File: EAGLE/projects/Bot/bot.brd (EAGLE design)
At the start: 124.3 x 90 mm, 17 parts, among them IC1 7805T, U3 ARDUINO_SHIELDLABEL

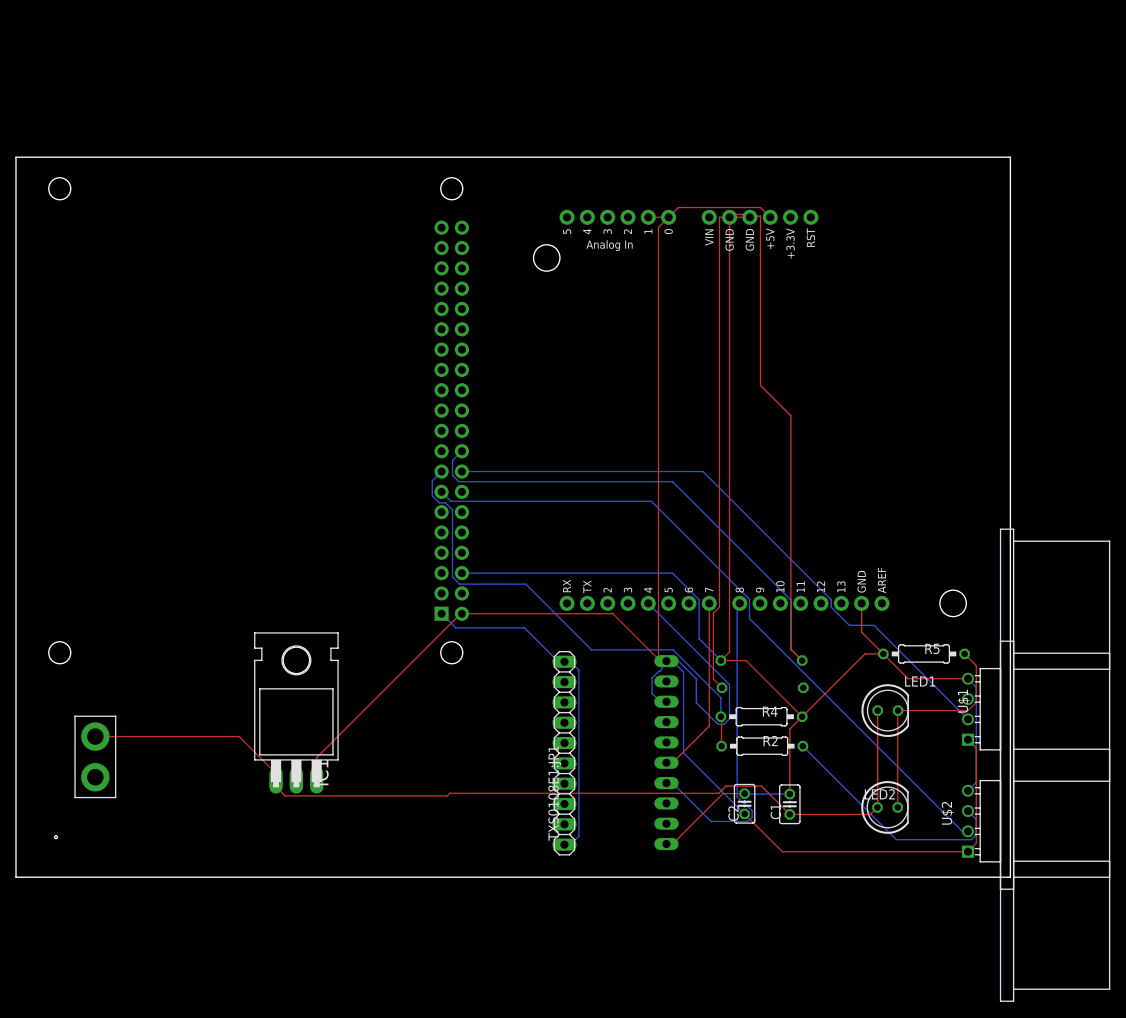
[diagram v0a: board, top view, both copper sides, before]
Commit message: Final PCB
PCB
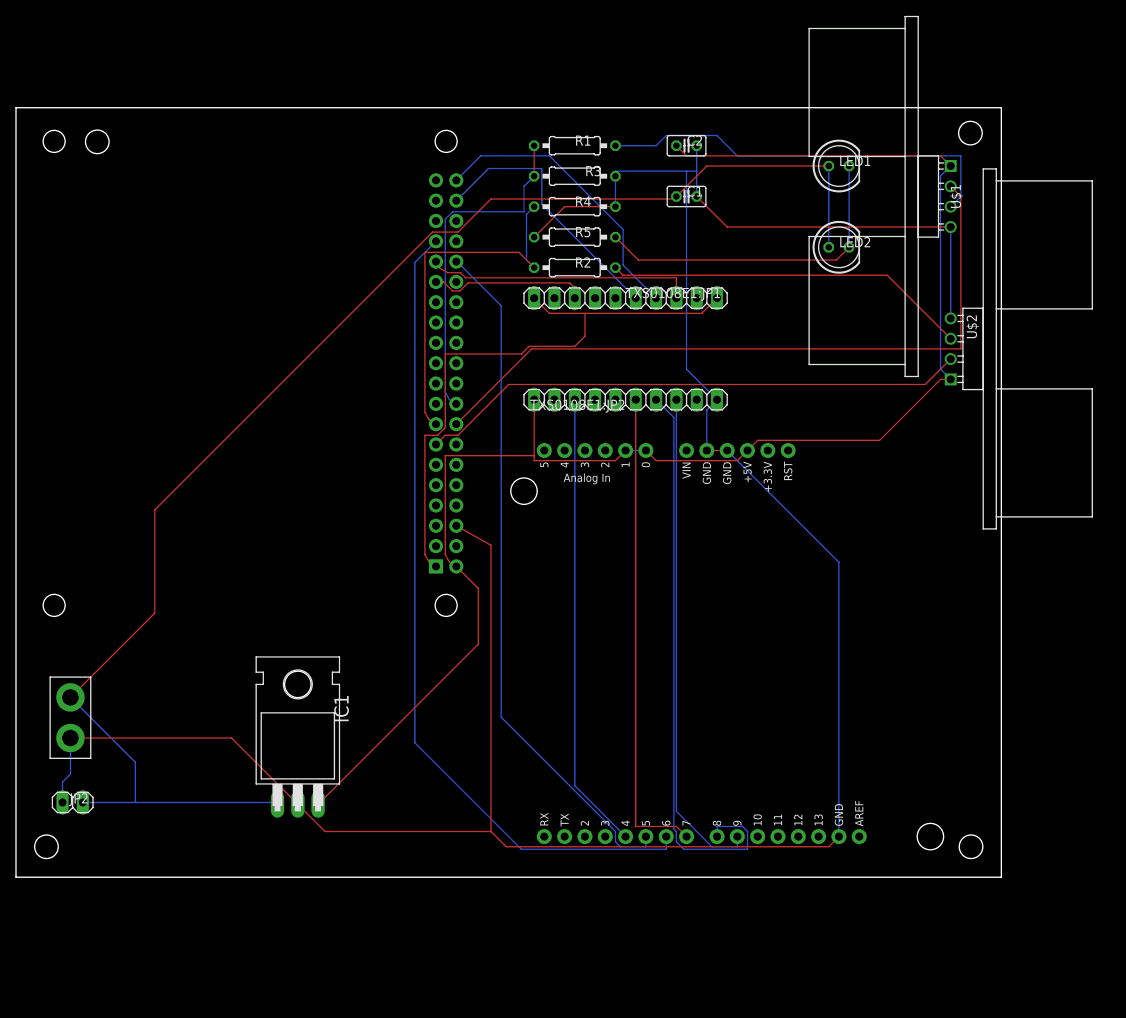
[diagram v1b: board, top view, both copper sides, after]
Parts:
- added JP2: (no value), pinhead:1X02
- R5: value 1k -> 10
- moved C2 82.6 mm to (83.8, 91.4), turned to 0 degrees
- moved C1 77.1 mm to (83.8, 85.1), turned to 0 degrees
- moved R1 71.7 mm to (69.8, 91.4), flipped to the top, turned to 0 degrees
- moved LED2 70.3 mm to (102.9, 78.7)
- moved LED1 68.3 mm to (102.9, 88.9)
- moved R5 68.0 mm to (69.8, 80.0)
- moved R4 67.9 mm to (69.8, 83.8)
- moved R3 64.9 mm to (69.8, 87.6), flipped to the top
- moved R2 64.2 mm to (69.8, 76.2)
- moved U$1 64.1 mm to (116.8, 85.1), turned to 270 degrees
- moved U$2 59.1 mm to (116.8, 66.0)
- moved TXS0108E1:JP1 57.4 mm to (76.2, 72.4), turned to 0 degrees
- moved TXS0108E1:JP2 44.4 mm to (76.2, 59.7), flipped to the top, turned to 180 degrees
- moved U3 29.3 mm to (120.7, 2.54)
- moved PI 5.96 mm to (1.27, 30.5)
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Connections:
- removed net S$1: IC1.2
- net 0: now also IC1.2, JP2.1, JP7.2
- net PWR+: now also JP2.2
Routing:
- net L_US_ECHO: track 183.1 -> 42.7 mm
- net 0: track 187.2 -> 322.5 mm
- net R_SPD: track 0.00 -> 102.3 mm
- net L_SPD: track 0.00 -> 86.1 mm
- net PWR+: track 116.3 -> 180.9 mm
- net N$16: track 0.00 -> 62.2 mm
- net N$1: track 0.00 -> 51.6 mm
- net N$14: track 22.6 -> 60.2 mm
- net L_BCK: track 0.00 -> 36.2 mm
- net R_BCK: track 0.00 -> 33.5 mm
- net L_FWD: track 0.00 -> 33.4 mm
- net N$15: track 40.6 -> 73.1 mm
- net PI_3V3: track 43.1 -> 74.8 mm
- net R_FWD: track 0.00 -> 19.9 mm
- net N$13: track 39.4 -> 57.2 mm
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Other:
- board size 124.3 x 90 mm -> 123.2 x 96.2 mm
